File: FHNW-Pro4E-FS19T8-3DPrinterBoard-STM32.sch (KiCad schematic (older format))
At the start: 31 parts, among them J101 Screw_Terminal_01x02, T101 BUK963R3-60E, U101 LM2675M-3.3, U102 LM2675M-5

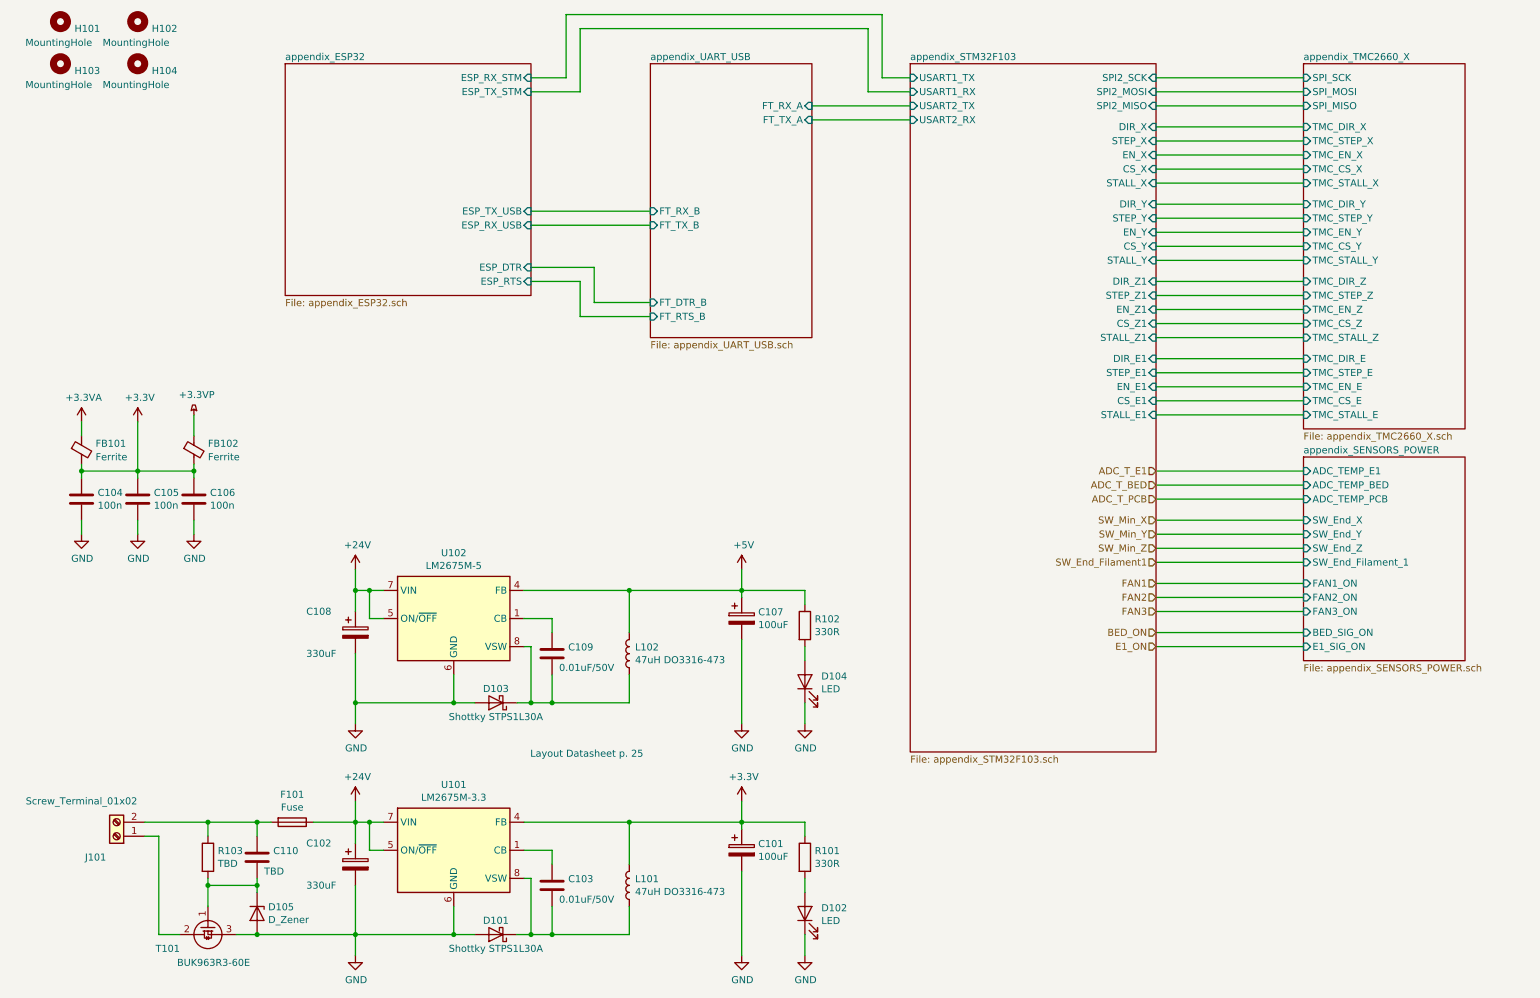
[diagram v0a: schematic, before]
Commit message: first layout draft without 40pin
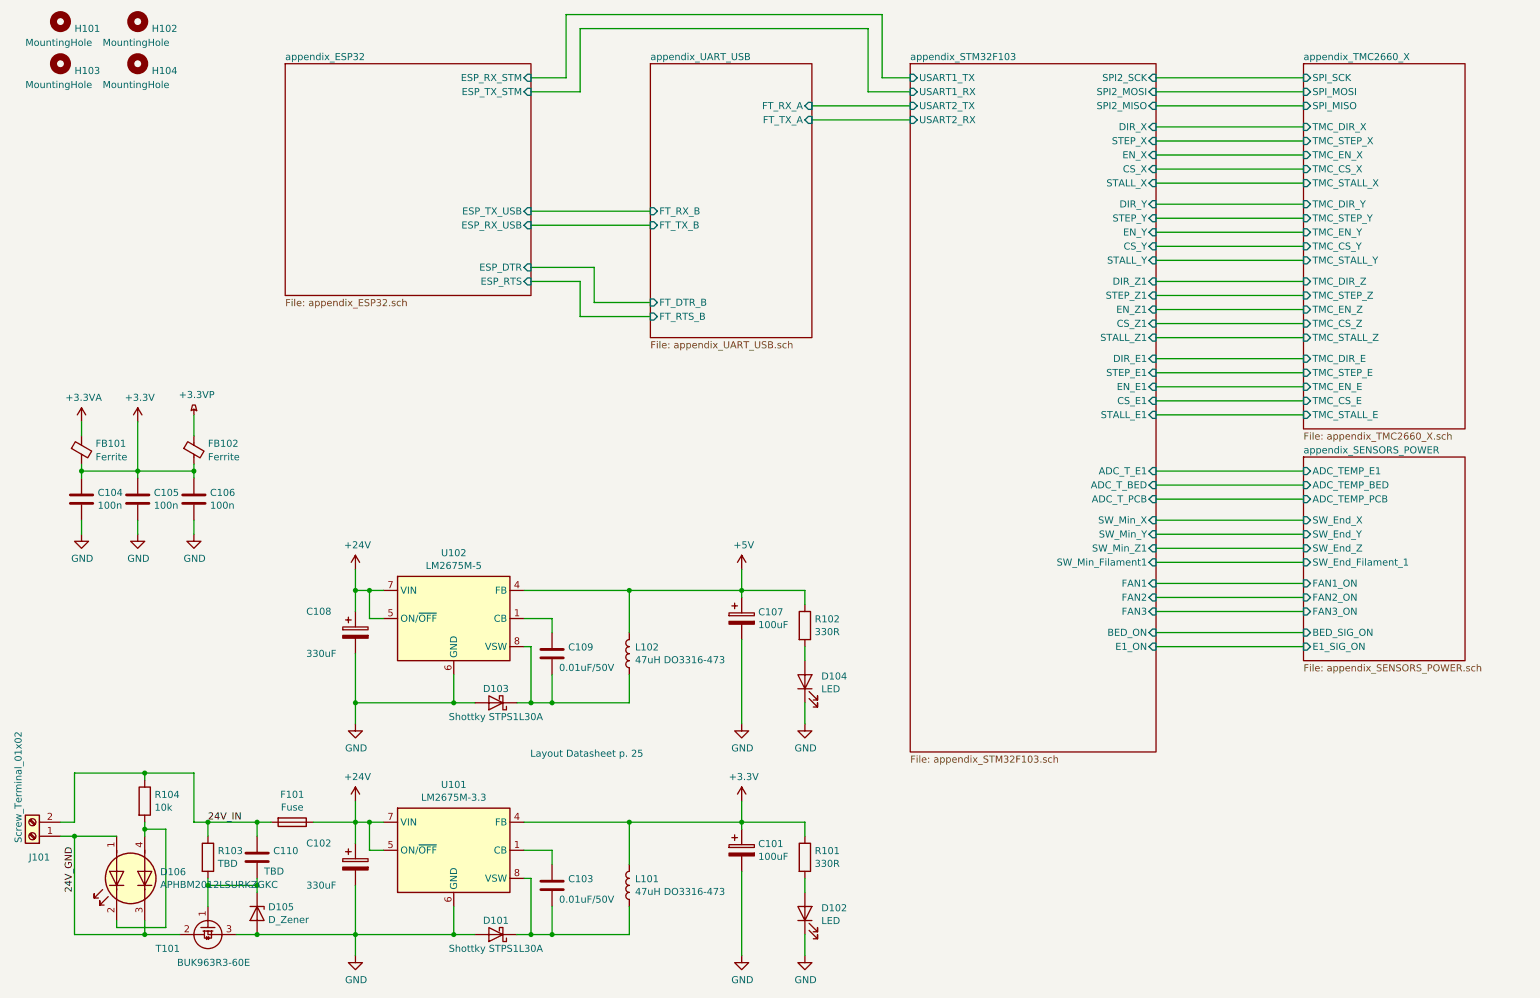
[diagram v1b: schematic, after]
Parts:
- added D106: APHBM2012LSURKZGKC, FHNW-Pro4E-FS19T8-Library:LED_Kingbright_SMD4_2.0x1.25, symbol FHNW-Pro4E-FS19T8-Library:APHBM2012LSURKZGKC
- added R104: 10k, Resistors_SMD:R_1206, symbol Device:R
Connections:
- net 24V_GND: now reaches J101.1 (Pin_1), T101.2
- net 24V_GND: now also D106.1 (A1), D106.3 (K2)
- net 24V_IN: now reaches C110.1, F101.2, J101.2 (Pin_2), R103.1
- net 24V_IN: now also R104.1
- new net: D106.2 (K1), D106.4 (A2), R104.2
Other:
- moved on the sheet: J101
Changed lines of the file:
@@
 F27 "CS_E1" I R 8650 3450 50
 F28 "STALL_E1" I R 8650 3550 50
+F29 "ADC_T_E1" I R 8650 3950 50
+F30 "ADC_T_BED" I R 8650 4050 50
+F31 "BED_ON" I R 8650 5100 50
+F32 "E1_ON" I R 8650 5200 50
+F33 "FAN1" I R 8650 4750 50
+F34 "FAN2" I R 8650 4850 50
+F35 "FAN3" I R 8650 4950 50
+F36 "ADC_T_PCB" I R 8650 4150 50
+F37 "SW_Min_X" I R 8650 4300 50
+F38 "SW_Min_Y" I R 8650 4400 50
+F39 "SW_Min_Z1" I R 8650 4500 50
+F40 "SW_Min_Filament1" I R 8650 4600 50
 $EndSheet
 $Sheet
@@
 L Connector:Screw_Terminal_01x02 J101
 U 1 1 5CD68AD6
-P 1250 6550
-F 0 "J101" H 1400 6700 50  0000 C CNN
-F 1 "Screw_Terminal_01x02" H 1500 6300 50  0000 C CNN
-F 2 "Connectors_Terminal_Blocks:TerminalBlock_Altech_AK300-2_P5.00mm" H 1250 6550 50  0001 C CNN
-F 3 "~" H 1250 6550 50  0001 C CNN
-	1    1250 6550
+P 650 6550
+F 0 "J101" H 600 6700 50  0000 C CNN
+F 1 "Screw_Terminal_01x02" V 750 6200 50  0000 C CNN
+F 2 "Connectors_Terminal_Blocks:TerminalBlock_Altech_AK300-2_P5.00mm" H 650 6550 50  0001 C CNN
+F 3 "~" H 650 6550 50  0001 C CNN
+	1    650  6550
 	-1   0    0    1
 $EndComp
@@
 $EndComp
 $Comp
-L Device:C C105
-U 1 1 5CC01495
-P 1400 4150
-F 0 "C105" H 1515 4196 50  0000 L CNN
-F 1 "100n" H 1515 4105 50  0000 L CNN
-F 2 "Capacitors_SMD:C_0603" H 1438 4000 50  0001 C CNN
-F 3 "~" H 1400 4150 50  0001 C CNN
-	1    1400 4150
-	1    0    0    -1
-$EndComp
-$Comp
 L power:GND #PWR0126
 U 1 1 5CC014A2
@@
 Wire Wire Line
 	9700 4950 8650 4950
-Text HLabel 8650 4050 0    50   Input ~ 0
-ADC_T_BED
-Text HLabel 8650 3950 0    50   Input ~ 0
-ADC_T_E1
-Text HLabel 8650 4300 0    50   Input ~ 0
-SW_Min_X
-Text HLabel 8650 4400 0    50   Input ~ 0
-SW_Min_Y
-Text HLabel 8650 4500 0    50   Input ~ 0
-SW_Min_Z
-Text HLabel 8650 4600 0    50   Input ~ 0
-SW_End_Filament1
-Text HLabel 8650 4750 0    50   Input ~ 0
-FAN1
-Text HLabel 8650 4850 0    50   Input ~ 0
-FAN2
-Text HLabel 8650 4950 0    50   Input ~ 0
-FAN3
-Text HLabel 8650 5100 0    50   Input ~ 0
-BED_ON
-Text HLabel 8650 5200 0    50   Input ~ 0
-E1_ON
 Wire Wire Line
 	4200 2600 4550 2600
@@
 Wire Wire Line
 	1900 6450 2250 6450
-Wire Wire Line
-	1450 6450 1900 6450
-Connection ~ 1900 6450
-Wire Wire Line
-	1700 7250 1550 7250
-Wire Wire Line
-	1550 7250 1550 6550
-Wire Wire Line
-	1550 6550 1450 6550
 $Comp
 L Device:D_Zener D105
@@
 	0    1    1    0
 $EndComp
-Text HLabel 8650 4150 0    50   Input ~ 0
-ADC_T_PCB
 $Sheet
 S 9700 3850 1150 1450
@@
 Wire Wire Line
 	9700 5200 8650 5200
+Text Label 950  6950 1    50   ~ 0
+24V_GND
+Text Label 1900 6450 0    50   ~ 0
+24V_IN
+$Comp
+L Device:R R104
+U 1 1 5CC041F6
+P 1450 6300
+F 0 "R104" H 1520 6346 50  0000 L CNN
+F 1 "10k" H 1520 6255 50  0000 L CNN
+F 2 "Resistors_SMD:R_1206" V 1380 6300 50  0001 C CNN
+F 3 "~" H 1450 6300 50  0001 C CNN
+	1    1450 6300
+	1    0    0    -1
+$EndComp
+$Comp
+L FHNW-Pro4E-FS19T8-Library:APHBM2012LSURKZGKC D106
+U 1 1 5CC0EDCA
+P 1350 6850
+F 0 "D106" V 1304 6640 50  0000 R CNN
+F 1 "APHBM2012LSURKZGKC" V 1395 6640 50  0000 R CNN
+F 2 "FHNW-Pro4E-FS19T8-Library:LED_Kingbright_SMD4_2.0x1.25" H 1380 6850 50  0001 C CNN
+F 3 "~" H 1380 6850 50  0001 C CNN
+	1    1350 6850
+	0    -1   1    0
+$EndComp
+Wire Wire Line
+	950  7250 950  6550
+Wire Wire Line
+	950  6550 850  6550
+Wire Wire Line
+	950  7250 1450 7250
+Wire Wire Line
+	1450 7150 1450 7250
+Connection ~ 1450 7250
+Wire Wire Line
+	1450 7250 1700 7250
+Wire Wire Line
+	950  6550 1250 6550
+Connection ~ 950  6550
+Wire Wire Line
+	1250 7150 1250 7200
+Wire Wire Line
+	1250 7200 1600 7200
+Wire Wire Line
+	1600 7200 1600 6500
+Wire Wire Line
+	1600 6500 1450 6500
+Wire Wire Line
+	1450 6500 1450 6550
+Wire Wire Line
+	850  6450 950  6450
+Wire Wire Line
+	950  6450 950  6100
+Wire Wire Line
+	950  6100 1450 6100
+Wire Wire Line
+	1800 6100 1800 6450
+Wire Wire Line
+	1800 6450 1900 6450
+Connection ~ 1900 6450
+Wire Wire Line
+	1450 6450 1450 6500
+Connection ~ 1450 6500
+Wire Wire Line
+	1450 6150 1450 6100
+Connection ~ 1450 6100
+Wire Wire Line
+	1450 6100 1800 6100
+$Comp
+L Device:C C105
+U 1 1 5CC01495
+P 1400 4150
+F 0 "C105" H 1515 4196 50  0000 L CNN
+F 1 "100n" H 1515 4105 50  0000 L CNN
+F 2 "Capacitors_SMD:C_0603" H 1438 4000 50  0001 C CNN
+F 3 "~" H 1400 4150 50  0001 C CNN
+	1    1400 4150
+	1    0    0    -1
+$EndComp
 $EndSCHEMATC
